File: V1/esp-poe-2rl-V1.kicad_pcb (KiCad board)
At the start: 4 copper layers, 88 x 45 mm, 95 parts, among them J1 USB_C_Receptacle_USB2.0, J2 RJ45 JACK, J3 1x2P 5,08mm, J4 1x2P 5,08mm, K1 G5NB-1A-E-DC5, K2 G5NB-1A-E-DC5, Q1 UMH3N, Q2 WPM2015-3/TR, Q3 LMUN2211LT1G, Q4 MMBT2222A, Q5 MMBT2222A, SW1 RESET, U1 TPS2376DDAR-H, U2 TX4138, U3 SY8089A1AAC, U4 CH340C, U5 ESP32-WROOM-32UE-N16, U6 LAN8710A, U7 SHT31-DIS

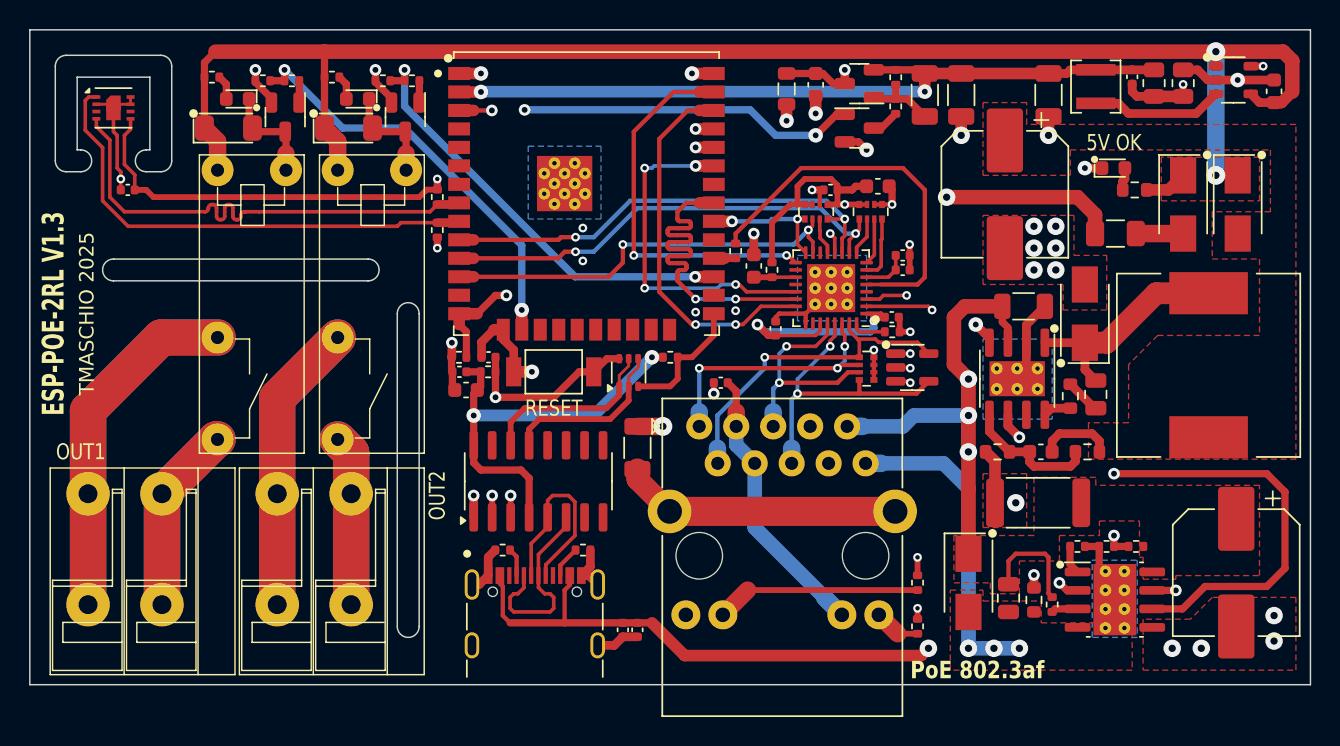
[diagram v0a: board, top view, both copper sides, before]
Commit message: V1.4
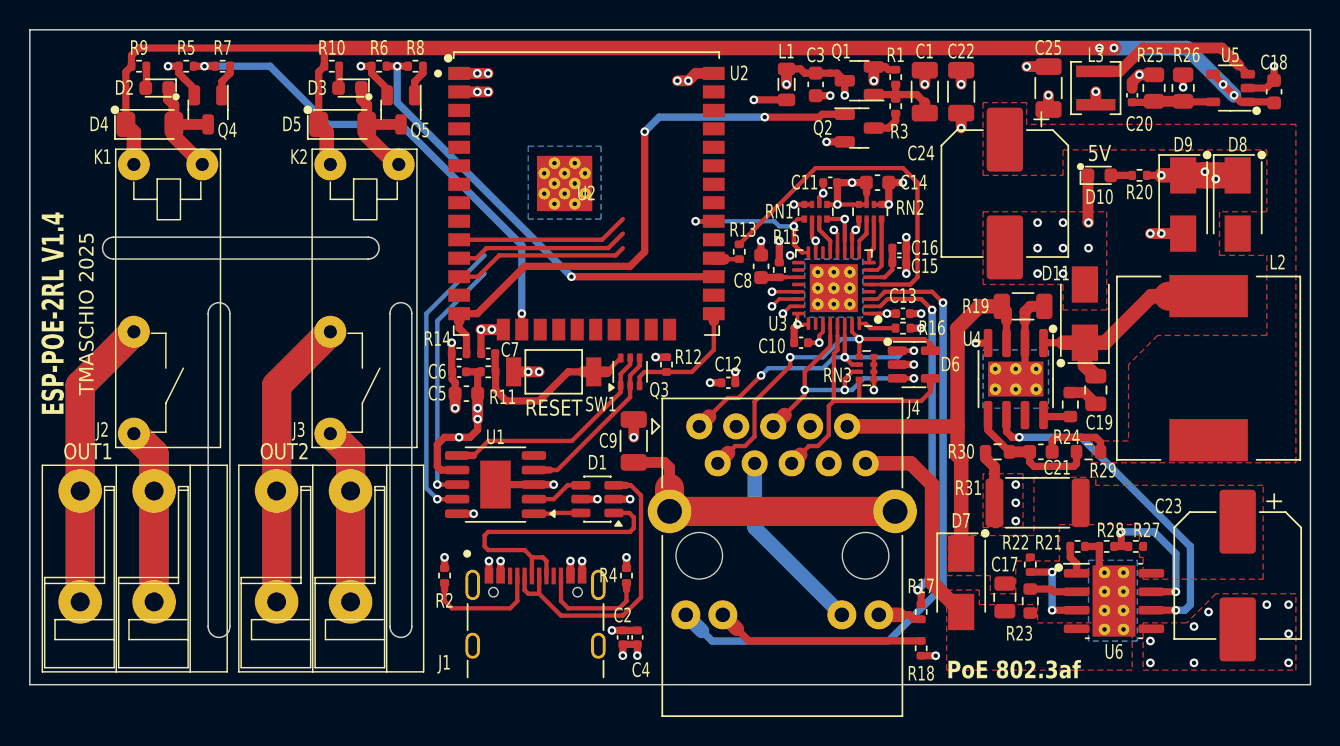
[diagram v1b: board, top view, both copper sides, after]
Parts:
- removed C26: 100nF/50V, Tales:C_0402_1005Metric
- removed F1: 500mA, Tales:Fuse_1206_3216Metric
- removed the R31 at (104.0, 84.8)
- removed R32: 2k2/62,5mW, Tales:R_0402_1005Metric
- removed the U4 at (110.9, 102.0)
- removed U7: SHT31-DIS, Tales:Sensirion_DFN-8-1EP_2.5x2.5mm_P0.5mm_EP1.1x1.7mm
- added D1: USBLC6-2SC6, Package_TO_SOT_SMD:SOT-23-6, F.Cu at (115.0, 103.2)
- added U1: CH340K, Package_SO:SSOP-10-1EP_3.9x4.9mm_P1mm_EP2.1x3.3mm, F.Cu at (108.0, 102.2)
- R1: renamed from R23; value 10k/62,5mW -> 10k
- R10: renamed from R30; value 680R/62,5mW -> 680R
- R11: renamed from R16; value 10k/62,5mW -> 10k
- R12: renamed from R17; value 10k/62,5mW -> 10k
- R13: renamed from R33; value 22R/62,5mW -> 22R
- R14: renamed from R18; value 10k/62,5mW -> 10k
- R15: renamed from R19; value 10k/62,5mW -> 10k
- R16: renamed from R20; value 12,1k/62,5mW -> 12,1k
- R17: renamed from R21; value 330R/62,5mW -> 330R
- R18: renamed from R22; value 330R/62,5mW -> 330R
- R2: renamed from R14; value 5,1k/62,5mW -> 5,1k
- R20: renamed from R11; value 820R/100mW -> 1k; footprint Tales:R_0603_1608Metric -> Tales:R_0402_1005Metric
- R21: renamed from R3; value 180k/62,5mW -> 180k
- R22: renamed from R5; value 30,1k/62,5mW -> 30,1k
- R27: renamed from R1; value 130k/62,5mW -> 130k
- R28: renamed from R2; value 10k/62,5mW -> 10k
- R3: renamed from R24; value 1k/62,5mW -> 1k
- R4: renamed from R15; value 5,1k/62,5mW -> 5,1k
- R5: renamed from R25; value 10k/62,5mW -> 10k
- R6: renamed from R28; value 10k/62,5mW -> 10k
- R7: renamed from R26; value 1k/62,5mW -> 1k
- R8: renamed from R29; value 1k/62,5mW -> 1k
- R9: renamed from R27; value 680R/62,5mW -> 680R
- RN1, RN2: value 4x2,2k/62,5mW -> 4x2,2k
- RN3: value 4x49,9R/62,5mW -> 4x49,9R
- moved K1 9.49 mm to (85.5, 89.5)
- moved K2 9.05 mm to (99.0, 89.5)
- moved D2 5.59 mm to (84.8, 75.0)
- moved D4 5.41 mm to (84.2, 77.5)
- moved R5 5.35 mm to (86.8, 73.5)
- moved Q4 5.32 mm to (88.2, 76.5)
- moved R9 5.07 mm to (83.5, 73.5)
- moved R7 4.86 mm to (89.2, 73.5)
- moved J3 4.72 mm to (95.5, 106.5)
- moved R18 4.52 mm to (137.2, 113.5), turned to -90 degrees
- moved J2 4.47 mm to (82.0, 106.5)
- moved R2 4.36 mm to (104.5, 108.5), turned to 90 degrees
- moved R4 3.46 mm to (117.0, 108.5), turned to 90 degrees
- moved R22 3.12 mm to (144.8, 107.8)
- moved C10 2.01 mm to (129.0, 92.5), turned to 180 degrees
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- renumbered C24 to C1, C16 to C10, C17 to C11, C23 to C12, C18 to C13, C19 to C14, C20 to C15, C21 to C16, C1 to C17, C6 to C18, C3 to C19, C10 to C2, C7 to C20, C4 to C21, C8 to C22, C2 to C23, C5 to C24, C9 to C25, C25 to C3, C11 to C4, C12 to C5, C13 to C6, C14 to C7, C15 to C8, C22 to C9, D5 to D10, D2 to D11, D7 to D2, D8 to D3, D9 to D4, D10 to D5, D1 to D7, D3 to D8, D4 to D9, J3 to J2, J4 to J3, J2 to J4, L3 to L1, L1 to L2, L2 to L3, Q2 to Q1, Q3 to Q2, Q1 to Q3, R7 to R19, R4 to R23, R8 to R24, R12 to R25, R13 to R26, R9 to R29, R10 to R30, R6 to R31, U5 to U2, U6 to U3, U2 to U4, U3 to U5, U1 to U6
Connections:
- net +3.3V renamed +3V3
- net +3.3VA renamed +3V3A
- net +3.3VLAN renamed +3V3LAN
- net /EMAC_CLK renamed /EMACCLK
- net /EMAC_MDC renamed /EMACMDC
- net /EMAC_MDIO renamed /EMACMDIO
- net /EMAC_RX renamed /EMACRX
- net /EMAC_RXD0 renamed /EMACRXD0
- net /EMAC_RXD1 renamed /EMACRXD1
- net /EMAC_TXD0 renamed /EMACTXD0
- net /EMAC_TXD1 renamed /EMACTXD1
- net /EMAC_TXEN renamed /EMACTXEN
- net /LED_G_K renamed /ETHLEDG
- net /LED_Y_A renamed /ETHLEDY
- net /RD+ renamed /ETHRXD+
- net /RD- renamed /ETHRXD-
- net /TD+ renamed /ETHTXD+
- net /TD- renamed /ETHTXD-
- net /USB_D+ renamed /USBCD+
- net /USB_D- renamed /USBCD-
- net Net-(C3-Pad1) renamed /POWER/5VBS
- net Net-(D10-A) renamed /OUT2CMD
- net Net-(D2-K) renamed /POWER/5VSW
- net Net-(D5-A) renamed /POWER/PWRON
- net Net-(D7-A) renamed /OUT1ON
- net Net-(D7-K) renamed /OUT1CMD
- net Net-(D8-A) renamed /OUT2ON
- net Net-(J1-CC1) renamed /USBCC1
- net Net-(J1-CC2) renamed /USBCC2
- net Net-(J2-LLED-) renamed /ETHLEDYK
- net Net-(J2-RLED-) renamed /ETHLEDGK
- net Net-(J2-SHIELD) renamed /ETHSH
- net Net-(J3-Pin_1) renamed /OUT1LN
- net Net-(J3-Pin_2) renamed /OUT1LD
- net Net-(J4-Pin_1) renamed /OUT2LN
- net Net-(J4-Pin_2) renamed /OUT2LD
- net Net-(Q1A-B1) renamed /UARTNDTR
- net Net-(Q1A-C1) renamed /ESPEN
- net Net-(Q1A-E1) renamed /UARTNRTS
- net Net-(Q1B-C2) renamed /ESPPROG
- net Net-(Q2-G) renamed /PHYPWRFET
- net Net-(Q3-C) renamed /PHYPWRBJT
- net Net-(Q4-B) renamed /OUT1BJT
- net Net-(Q5-B) renamed /OUT2BJT
- net Net-(R7-Pad2) renamed /POWER/ILIM
- net Net-(RN1-R3.1) renamed /EMACRXD4
- net Net-(RN2-R2.1) renamed /EMACRXD2
- net Net-(RN2-R3.1) renamed /EMACRXD3
- net Net-(RN2-R4.1) renamed /EMACRXCLK
- net Net-(U1-CLASS) renamed /POWER/RCLASS
- net Net-(U1-DET) renamed /POWER/RDET
- net Net-(U1-ILIM) renamed /POWER/RILIM
- net Net-(U1-UVLO) renamed /POWER/VTAP
- net Net-(U2-BS) renamed /POWER/BS
- net Net-(U2-FB) renamed /POWER/5VREF
- net Net-(U3-FB) renamed /POWER/3V3REF
- net Net-(U3-LX) renamed /POWER/3V3SW
- net Net-(U5-IO17) renamed /EMACGPIO
- net Net-(U6-RBIAS) renamed /RBIAS
- net Net-(U6-VDDCR) renamed /VDDCR
- net Net-(U6-~{RST}) renamed /PHYNRST
- net PHY_PWR renamed PHYPWR
- net PoE+ renamed POE+
- net PoE- renamed POE-
- C2 pad 1: Net-(C10-Pad1) -> 5VUSB
- C4 pad 1: Net-(C10-Pad1) -> 5VUSB
- J1 pad A4: Net-(C10-Pad1) -> 5VUSB
- J1 pad A9: Net-(C10-Pad1) -> 5VUSB
- J1 pad B4: Net-(C10-Pad1) -> 5VUSB
- J1 pad B9: Net-(C10-Pad1) -> 5VUSB
- U2 pad 34: Net-(U4-TXD) -> /UARTTXD
- U2 pad 35: Net-(U4-RXD) -> /UARTRXD
- U2 pad 8: I2C_SCL -> unconnected-(U2-IO32-Pad8)
- U2 pad 9: I2C_SDA -> unconnected-(U2-IO33-Pad9)
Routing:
- net +3V3: track 139.4 -> 37.2 mm, vias 6 -> 13
- net Net-(C10-Pad1): track 81.0 -> 0.00 mm, vias 2 -> 0
- net 5VUSB: track 3.25 -> 80.1 mm, vias 0 -> 6
- net +3V3A: track 63.2 -> 25.3 mm, vias 4 -> 5
- net Net-(U4-TXD): track 34.5 -> 0.00 mm, vias 2 -> 0
- net I2C_SDA: track 33.5 -> 0.00 mm
- net I2C_SCL: track 33.4 -> 0.00 mm
- net Net-(U4-RXD): track 33.2 -> 0.00 mm, vias 2 -> 0
- net /EMACMDC: track 26.5 -> 0.00 mm, vias 2 -> 1
- net /EMACTXD1: track 25.9 -> 1.27 mm, vias 2 -> 1
- net /EMACTXD0: track 25.8 -> 2.02 mm, vias 2 -> 1
- net /EMACTXEN: track 23.7 -> 1.81 mm, vias 4 -> 1
- net /ESPEN: track 34.4 -> 12.6 mm, vias 2 -> 0
- net /UARTRXD: track 0.00 -> 20.1 mm, vias 0 -> 1
- net /EMACRXD1: track 32.0 -> 14.5 mm, vias 2 -> 1
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- added copper zone on In2.Cu, net +3V3
- added copper zone on In2.Cu, net +3V3A
- added copper zone on In2.Cu, net +3V3LAN
- added copper zone on In2.Cu, net +5V
- added copper zone on In1.Cu, net POE-
- added copper zone on In2.Cu, net POE-
- removed copper zone on F.Cu, net +5V
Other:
- outline, holes or cut-outs redrawn
- rule pad_to_mask_clearance: 0 -> 0.1
- board text added: "5V"
- board text added: "ESP-POE-2RL V1.4"
- board text removed: "5V OK"
- board text removed: "ESP-POE-2RL V1.3"
